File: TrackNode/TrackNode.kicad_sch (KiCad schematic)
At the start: 15 parts, among them J1 Conn_01x04, J2 Conn_01x02, U1 TLV493D-A1B6, U2 LIS2DTW12

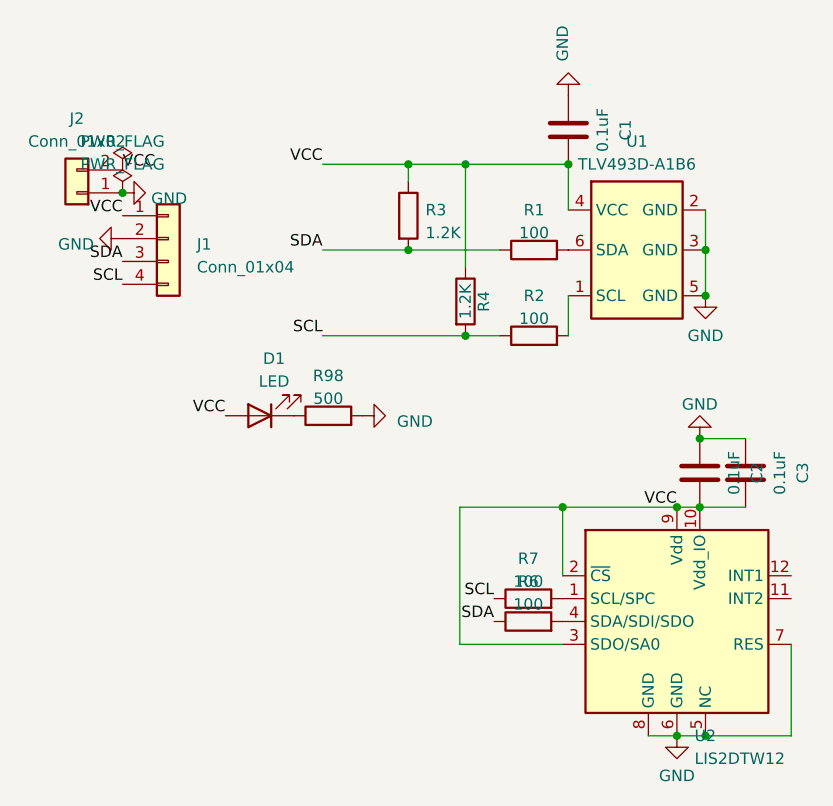
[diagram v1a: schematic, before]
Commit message: Finalized CAD files and configurations
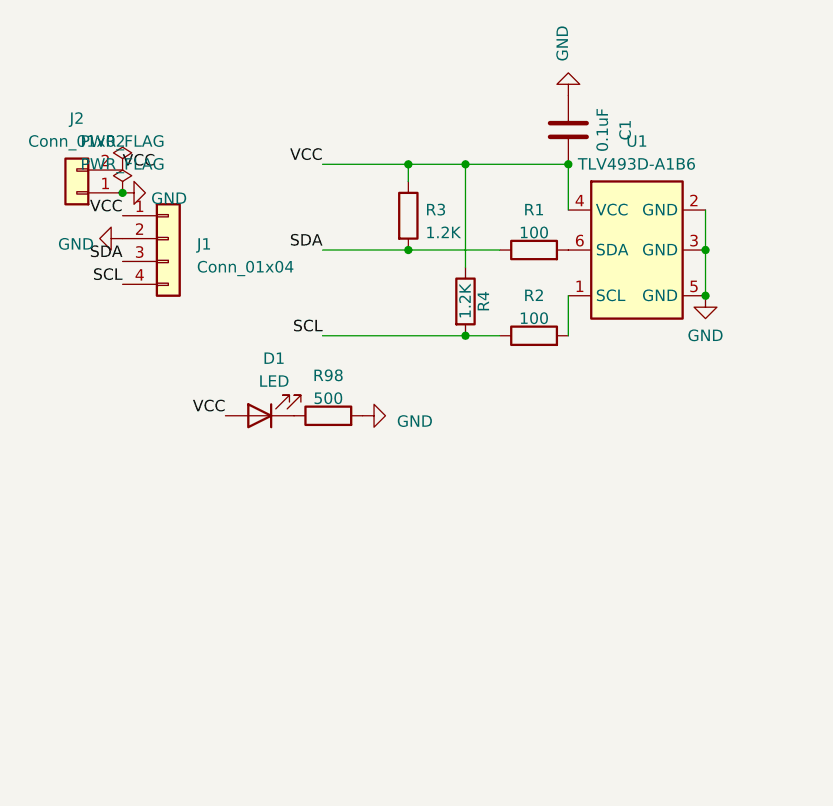
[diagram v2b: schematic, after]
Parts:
- removed C2, C3: 0.1uF, Capacitor_SMD:C_0402_1005Metric, symbol Device:C
- removed R6, R7: 100, Resistor_SMD:R_0402_1005Metric, symbol Device:R
- removed U2: LIS2DTW12, Package_LGA:LGA-12_2x2mm_P0.5mm, symbol Touchstone:LIS2DTW12
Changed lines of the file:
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@@
   (junction (at 92.075 37.465) (diameter 0) (color 0 0 0 0)
   )
-  (junction (at 88.9 91.44) (diameter 0) (color 0 0 0 0)
-  )
   (junction (at 65.405 46.99) (diameter 0) (color 0 0 0 0)
   )
-  (junction (at 88.9 66.04) (diameter 0) (color 0 0 0 0)
-  )
-  (junction (at 92.075 91.44) (diameter 0) (color 0 0 0 0)
-  )
   (junction (at 27.305 31.115) (diameter 0) (color 0 0 0 0)
   )
-  (junction (at 76.2 66.04) (diameter 0) (color 0 0 0 0)
-  )
   (junction (at 59.055 37.465) (diameter 0) (color 0 0 0 0)
   )
@@
   (junction (at 76.835 27.94) (diameter 0) (color 0 0 0 0)
   )
-  (junction (at 91.44 58.42) (diameter 0) (color 0 0 0 0)
-  )
-  (junction (at 91.44 66.04) (diameter 0) (color 0 0 0 0)
-  )
   (junction (at 65.405 27.94) (diameter 0) (color 0 0 0 0)
   )
@@
     (stroke (width 0) (type default))
   )
-  (wire (pts (xy 92.075 91.44) (xy 101.6 91.44))
-    (stroke (width 0) (type default))
-  )
   (wire (pts (xy 49.53 46.99) (xy 65.405 46.99))
     (stroke (width 0) (type default))
   )
-  (wire (pts (xy 76.2 66.04) (xy 88.9 66.04))
-    (stroke (width 0) (type default))
-  )
-  (wire (pts (xy 91.44 66.04) (xy 96.52 66.04))
-    (stroke (width 0) (type default))
-  )
   (wire (pts (xy 49.53 27.94) (xy 59.055 27.94))
     (stroke (width 0) (type default))
   )
-  (wire (pts (xy 85.725 91.44) (xy 88.9 91.44))
-    (stroke (width 0) (type default))
-  )
-  (wire (pts (xy 64.77 66.04) (xy 76.2 66.04))
-    (stroke (width 0) (type default))
-  )
-  (wire (pts (xy 76.2 81.28) (xy 64.77 81.28))
-    (stroke (width 0) (type default))
-  )
   (wire (pts (xy 92.075 37.465) (xy 92.075 42.545))
     (stroke (width 0) (type default))
@@
     (stroke (width 0) (type default))
   )
-  (wire (pts (xy 64.77 81.28) (xy 64.77 66.04))
-    (stroke (width 0) (type default))
-  )
-  (wire (pts (xy 101.6 81.28) (xy 101.6 91.44))
-    (stroke (width 0) (type default))
-  )
-  (wire (pts (xy 88.9 66.04) (xy 91.44 66.04))
-    (stroke (width 0) (type default))
-  )
   (wire (pts (xy 76.835 27.94) (xy 76.835 33.02))
     (stroke (width 0) (type default))
@@
     (stroke (width 0) (type default))
   )
-  (wire (pts (xy 76.2 73.66) (xy 76.2 66.04))
-    (stroke (width 0) (type default))
-  )
   (wire (pts (xy 59.055 37.465) (xy 69.215 37.465))
     (stroke (width 0) (type default))
@@
     (stroke (width 0) (type default))
   )
-  (wire (pts (xy 88.9 91.44) (xy 92.075 91.44))
-    (stroke (width 0) (type default))
-  )
   (wire (pts (xy 59.055 27.94) (xy 59.055 29.845))
     (stroke (width 0) (type default))
   )
-  (wire (pts (xy 91.44 58.42) (xy 96.52 58.42))
-    (stroke (width 0) (type default))
-  )
   (wire (pts (xy 59.055 27.94) (xy 65.405 27.94))
     (stroke (width 0) (type default))
@@
     (stroke (width 0) (type default))
   )
-  (label "SCL" (at 68.58 76.2 180) (fields_autoplaced)
-    (effects (font (size 1.27 1.27)) (justify right bottom))
-  )
-  (label "SDA" (at 68.58 78.74 180) (fields_autoplaced)
-    (effects (font (size 1.27 1.27)) (justify right bottom))
-  )
   (label "SDA" (at 49.53 37.465 180) (fields_autoplaced)
     (effects (font (size 1.27 1.27)) (justify right bottom))
@@
   )
   (label "SDA" (at 27.305 38.735 180) (fields_autoplaced)
-    (effects (font (size 1.27 1.27)) (justify right bottom))
-  )
-  (label "VCC" (at 88.9 66.04 180) (fields_autoplaced)
     (effects (font (size 1.27 1.27)) (justify right bottom))
   )
@@
     )
   )
-  (symbol (lib_id "Device:R") (at 72.39 76.2 90) (unit 1)
-    (in_bom yes) (on_board yes) (dnp no) (fields_autoplaced)
-    (property "Reference" "R7" (at 72.39 71.755 90)
-      (effects (font (size 1.27 1.27)))
-    )
-    (property "Value" "100" (at 72.39 74.295 90)
-      (effects (font (size 1.27 1.27)))
-    )
-    (property "Footprint" "Resistor_SMD:R_0402_1005Metric" (at 72.39 77.978 90)
-      (effects (font (size 1.27 1.27)) hide)
-    )
-    (property "Datasheet" "~" (at 72.39 76.2 0)
-      (effects (font (size 1.27 1.27)) hide)
-    )
-    (pin "1")
-    (pin "2")
-    (instances
-      (project "TrackNode"
-        (path "/1a22a45d-0453-4b94-9e49-dc92af99da64"
-          (reference "R7") (unit 1)
-        )
-      )
-    )
-  )
   (symbol (lib_id "power:GND") (at 27.305 31.115 90) (unit 1)
     (in_bom yes) (on_board yes) (dnp no) (fields_autoplaced)
@@
         (path "/1a22a45d-0453-4b94-9e49-dc92af99da64"
           (reference "#PWR07") (unit 1)
-        )
-      )
-    )
-  )
-  (symbol (lib_id "Device:R") (at 72.39 78.74 90) (unit 1)
-    (in_bom yes) (on_board yes) (dnp no) (fields_autoplaced)
-    (property "Reference" "R6" (at 72.39 74.295 90)
-      (effects (font (size 1.27 1.27)))
-    )
-    (property "Value" "100" (at 72.39 76.835 90)
-      (effects (font (size 1.27 1.27)))
-    )
-    (property "Footprint" "Resistor_SMD:R_0402_1005Metric" (at 72.39 80.518 90)
-      (effects (font (size 1.27 1.27)) hide)
-    )
-    (property "Datasheet" "~" (at 72.39 78.74 0)
-      (effects (font (size 1.27 1.27)) hide)
-    )
-    (pin "1")
-    (pin "2")
-    (instances
-      (project "TrackNode"
-        (path "/1a22a45d-0453-4b94-9e49-dc92af99da64"
-          (reference "R6") (unit 1)
-        )
-      )
-    )
-  )
-  (symbol (lib_id "Device:C") (at 96.52 62.23 0) (unit 1)
-    (in_bom yes) (on_board yes) (dnp no) (fields_autoplaced)
-    (property "Reference" "C3" (at 102.87 62.23 90)
-      (effects (font (size 1.27 1.27)))
-    )
-    (property "Value" "0.1uF" (at 100.33 62.23 90)
-      (effects (font (size 1.27 1.27)))
-    )
-    (property "Footprint" "Capacitor_SMD:C_0402_1005Metric" (at 97.4852 66.04 0)
-      (effects (font (size 1.27 1.27)) hide)
-    )
-    (property "Datasheet" "~" (at 96.52 62.23 0)
-      (effects (font (size 1.27 1.27)) hide)
-    )
-    (pin "1")
-    (pin "2")
-    (instances
-      (project "TrackNode"
-        (path "/1a22a45d-0453-4b94-9e49-dc92af99da64"
-          (reference "C3") (unit 1)
-        )
-      )
-    )
-  )
-  (symbol (lib_id "Device:C") (at 91.44 62.23 0) (unit 1)
-    (in_bom yes) (on_board yes) (dnp no) (fields_autoplaced)
-    (property "Reference" "C2" (at 97.79 62.23 90)
-      (effects (font (size 1.27 1.27)))
-    )
-    (property "Value" "0.1uF" (at 95.25 62.23 90)
-      (effects (font (size 1.27 1.27)))
-    )
-    (property "Footprint" "Capacitor_SMD:C_0402_1005Metric" (at 92.4052 66.04 0)
-      (effects (font (size 1.27 1.27)) hide)
-    )
-    (property "Datasheet" "~" (at 91.44 62.23 0)
-      (effects (font (size 1.27 1.27)) hide)
-    )
-    (pin "1")
-    (pin "2")
-    (instances
-      (project "TrackNode"
-        (path "/1a22a45d-0453-4b94-9e49-dc92af99da64"
-          (reference "C2") (unit 1)
         )
       )
@@
     )
   )
-  (symbol (lib_id "power:GND") (at 91.44 58.42 180) (unit 1)
-    (in_bom yes) (on_board yes) (dnp no) (fields_autoplaced)
-    (property "Reference" "#PWR06" (at 91.44 52.07 0)
-      (effects (font (size 1.27 1.27)) hide)
-    )
-    (property "Value" "GND" (at 91.44 54.61 0)
-      (effects (font (size 1.27 1.27)))
-    )
-    (property "Footprint" "" (at 91.44 58.42 0)
-      (effects (font (size 1.27 1.27)) hide)
-    )
-    (property "Datasheet" "" (at 91.44 58.42 0)
-      (effects (font (size 1.27 1.27)) hide)
-    )
-    (pin "1")
-    (instances
-      (project "TrackNode"
-        (path "/1a22a45d-0453-4b94-9e49-dc92af99da64"
-          (reference "#PWR06") (unit 1)
-        )
-      )
-    )
-  )
   (symbol (lib_id "Device:R") (at 73.025 37.465 90) (unit 1)
     (in_bom yes) (on_board yes) (dnp no) (fields_autoplaced)
@@
     )
   )
-  (symbol (lib_id "Touchstone:LIS2DTW12") (at 88.9 78.74 0) (unit 1)
-    (in_bom yes) (on_board yes) (dnp no) (fields_autoplaced)
-    (property "Reference" "U2" (at 90.8559 91.44 0)
-      (effects (font (size 1.27 1.27)) (justify left))
-    )
-    (property "Value" "LIS2DTW12" (at 90.8559 93.98 0)
-      (effects (font (size 1.27 1.27)) (justify left))
-    )
-    (property "Footprint" "Package_LGA:LGA-12_2x2mm_P0.5mm" (at 119.38 86.36 0)
-      (effects (font (size 1.27 1.27)) hide)
-    )
-    (property "Datasheet" "https://www.st.com/resource/en/datasheet/lis2dtw12.pdf" (at 127 88.9 0)
-      (effects (font (size 1.27 1.27)) hide)
-    )
-    (pin "1")
-    (pin "10")
-    (pin "11")
-    (pin "12")
-    (pin "2")
-    (pin "3")
-    (pin "4")
-    (pin "5")
-    (pin "6")
-    (pin "7")
-    (pin "8")
-    (pin "9")
-    (instances
-      (project "TrackNode"
-        (path "/1a22a45d-0453-4b94-9e49-dc92af99da64"
-          (reference "U2") (unit 1)
-        )
-      )
-    )
-  )
   (symbol (lib_id "Device:LED") (at 42.545 55.88 180) (unit 1)
     (in_bom yes) (on_board yes) (dnp no) (fields_autoplaced)
@@
         )
       )
-    )
-  )
-  (symbol (lib_id "power:GND") (at 88.9 91.44 0) (unit 1)
-    (in_bom yes) (on_board yes) (dnp no) (fields_autoplaced)
-    (property "Reference" "#PWR05" (at 88.9 97.79 0)
-      (effects (font (size 1.27 1.27)) hide)
-    )
-    (property "Value" "GND" (at 88.9 95.885 0)
-      (effects (font (size 1.27 1.27)))
-    )
-    (property "Footprint" "" (at 88.9 91.44 0)
-      (effects (font (size 1.27 1.27)) hide)
-    )
-    (property "Datasheet" "" (at 88.9 91.44 0)
-      (effects (font (size 1.27 1.27)) hide)
-    )
-    (pin "1")
-    (instances
-      (project "TrackNode"
-        (path "/1a22a45d-0453-4b94-9e49-dc92af99da64"
-          (reference "#PWR05") (unit 1)
-        )
-      )
-      (project "BusChain"
-        (path "/a3c96221-c538-4784-bbfe-f272329e4c12"
-          (reference "#PWR026") (unit 1)
-        )
-      )

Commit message: Fixed direction of TrackNode pin header
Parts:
- J2: footprint Connector_PinHeader_2.54mm:PinHeader_1x02_P2.54mm_Vertical -> Connector_PinHeader_2.54mm:PinHeader_1x02_P2.54mm_Horizontal
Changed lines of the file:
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@@
       (effects (font (size 1.27 1.27)))
     )
-    (property "Footprint" "Connector_PinHeader_2.54mm:PinHeader_1x02_P2.54mm_Vertical" (at 22.225 31.115 0)
+    (property "Footprint" "Connector_PinHeader_2.54mm:PinHeader_1x02_P2.54mm_Horizontal" (at 22.225 31.115 0)
       (effects (font (size 1.27 1.27)) hide)
     )
